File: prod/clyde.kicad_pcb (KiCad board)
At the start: 2 copper layers, 114.3 x 83.3 mm, 60 parts

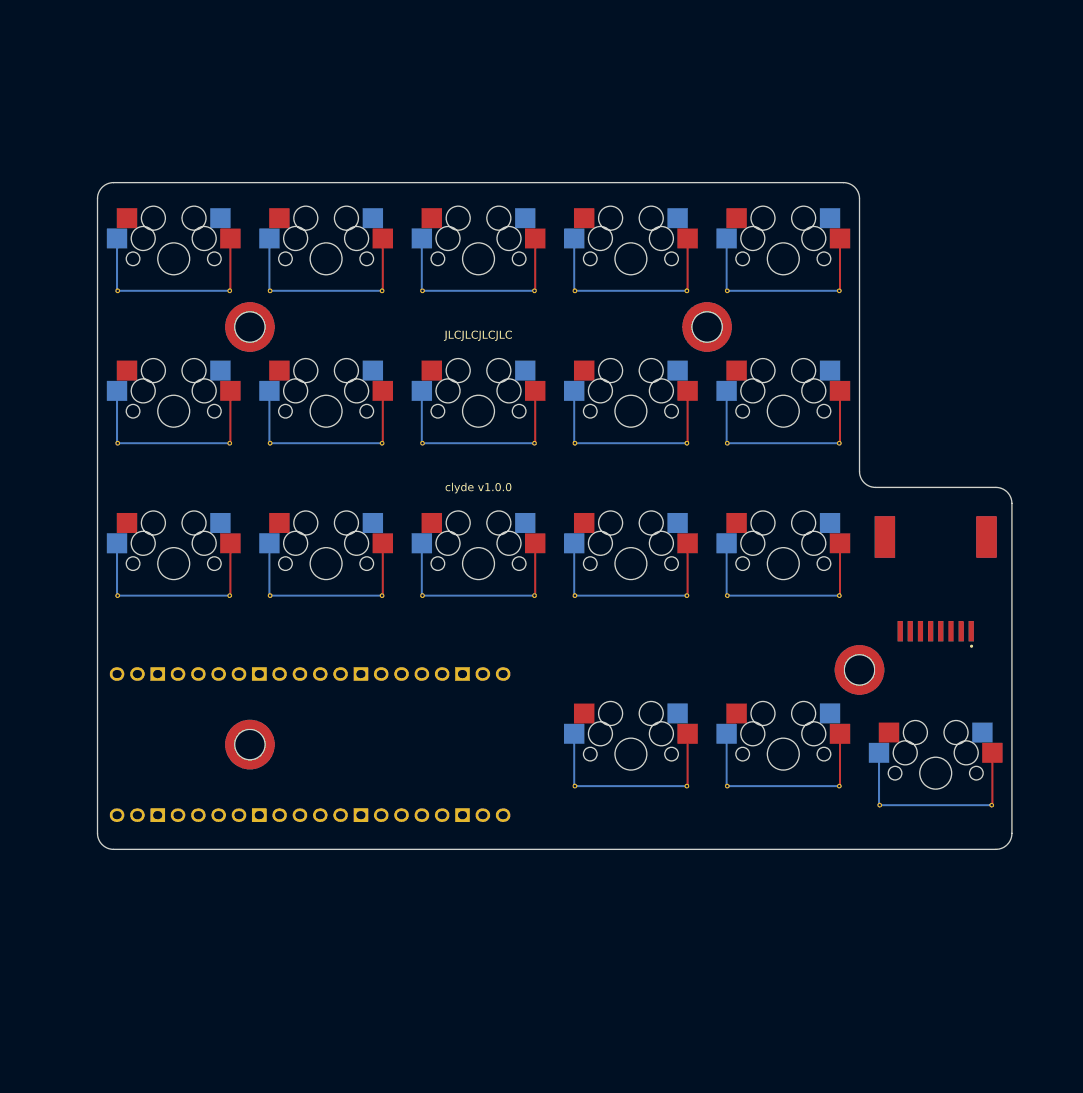
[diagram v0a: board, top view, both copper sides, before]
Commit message: finish routing
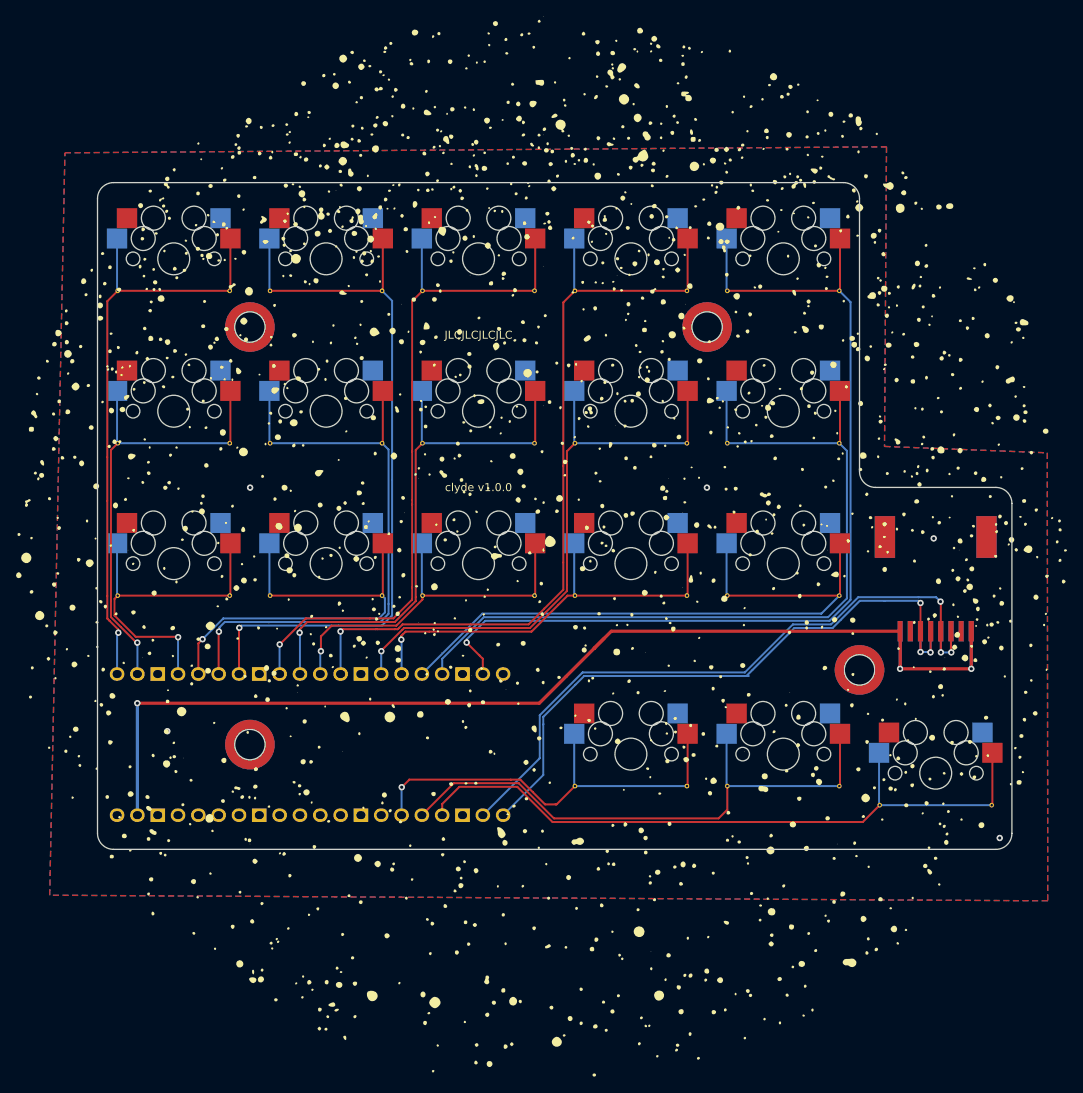
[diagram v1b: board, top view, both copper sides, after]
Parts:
- added G***: LOGO, main:north-sky-silk, F.Cu at (198.6, 150.8)
- added G***: LOGO, main:north-sky-silk, B.Cu at (198.5, 150.8)
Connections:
- U0 pad 5: matrix_ring_top -> matrix_ring_bottom
- U0 pad 7: matrix_ring_bottom -> matrix_ring_top
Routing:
- net VSYS: track 0.00 -> 142.6 mm, vias 0 -> 3
- net matrix_inner_top: track 27.2 -> 121.6 mm, vias 0 -> 1
- net GP17: track 0.00 -> 87.5 mm, vias 0 -> 3
- net GP16: track 0.00 -> 84.4 mm, vias 0 -> 3
- net matrix_inner_home: track 27.2 -> 102.6 mm
- net matrix_index_top: track 27.2 -> 100.4 mm, vias 0 -> 1
- net matrix_ring_top: track 27.2 -> 93.8 mm, vias 0 -> 1
- net matrix_middle_top: track 27.2 -> 88.9 mm, vias 0 -> 1
- net thumb_far_mods: track 27.2 -> 86.8 mm
- net matrix_inner_bottom: track 27.2 -> 83.4 mm
- net matrix_ring_home: track 27.2 -> 76.5 mm, vias 0 -> 1
- net matrix_pinky_top: track 27.2 -> 76.2 mm, vias 0 -> 1
- net matrix_index_home: track 27.2 -> 75.3 mm, vias 0 -> 1
- net thumb_middle_mods: track 27.2 -> 72.2 mm
- net matrix_middle_home: track 27.2 -> 68.8 mm, vias 0 -> 1
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- added copper zone on B.Cu, net GND
- added copper zone on F.Cu, net GND
